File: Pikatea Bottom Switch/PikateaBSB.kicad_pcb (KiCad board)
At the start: 2 copper layers, 125.6 x 26 mm, 19 parts, among them J1 Conn_01x16, J2 Conn_01x03, J3 Conn_01x03, U1 AMS1117-3.3, U2 74LVC125APW,118

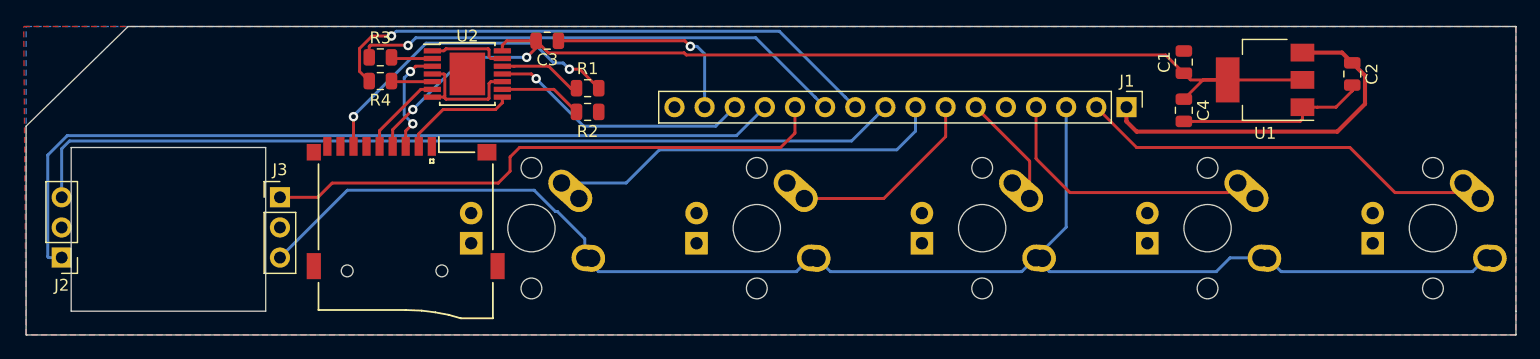
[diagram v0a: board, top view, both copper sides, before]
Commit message: Update Doughter board
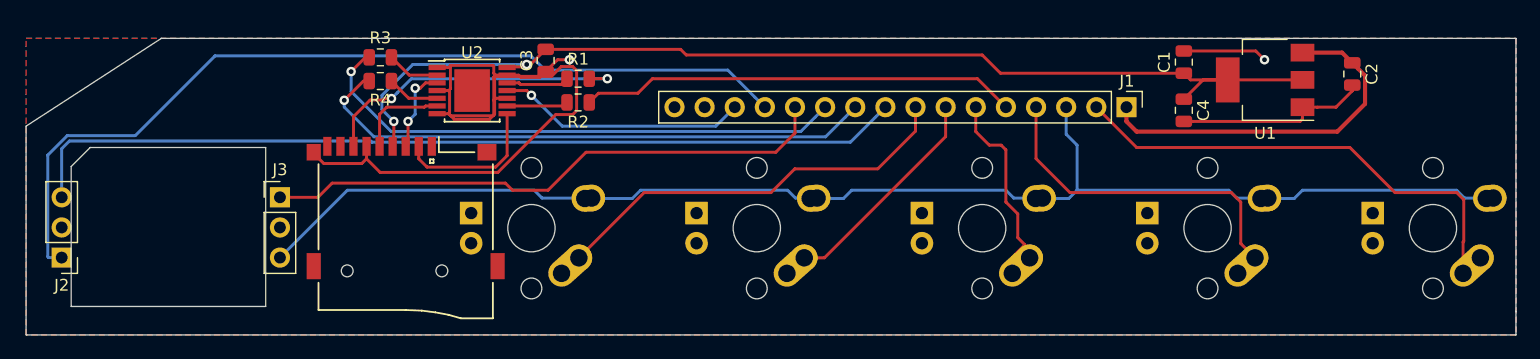
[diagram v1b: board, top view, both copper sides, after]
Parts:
- MX1, MX2, MX3, MX4, MX5: moved to B.Cu
- moved C3 1.67 mm to (158.6, 45.5), turned to 270 degrees
- moved U2 1.46 mm to (152.4, 48.0)
- moved R1 1.13 mm to (161.3, 47.0)
- moved R2 1.13 mm to (161.3, 49.0)
- turned MX1 to 90 degrees
- turned MX2 to 90 degrees
- turned MX3 to 90 degrees
- turned MX4 to 90 degrees
- turned MX5 to 90 degrees
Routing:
- net GND: track 50.6 -> 95.2 mm, vias 1 -> 2
- net /CS: track 0.00 -> 36.9 mm
- net /D9: track 9.58 -> 18.4 mm
- net /A0: track 123.8 -> 115.2 mm
- net /D7: track 34.2 -> 42.1 mm
- net /D8: track 16.6 -> 22.3 mm
- net /D5: track 22.9 -> 28.3 mm
- net /MOSI: track 42.1 -> 45.9 mm
- net /D3: track 71.9 -> 75.5 mm
- net /D6: track 33.7 -> 36.8 mm
- net Net-(U2-Pad8): track 9.66 -> 12.7 mm
- net Net-(U2-Pad3): track 9.39 -> 7.27 mm
- net Net-(R2-Pad2): track 7.04 -> 5.17 mm
- net Net-(R1-Pad1): track 7.02 -> 5.31 mm
- net Net-(R3-Pad2): track 3.49 -> 4.61 mm
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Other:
- board size 125.6 x 26 mm -> 125.6 x 25 mm
